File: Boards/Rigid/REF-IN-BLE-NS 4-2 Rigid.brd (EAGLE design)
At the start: 44 x 96.5 mm, 82 parts, among them U1 NRF52832_10QFN48, U2 AEM10941, X1 32 MHz, X2 32.768 kHz

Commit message: Removed internal pullups, changed xtal caps 12pf
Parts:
- C1, C17, C18, C2: value 9pF -> 12pF
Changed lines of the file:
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@@
 <elements>
 <element name="AE1" library="00_PF_Nordic" package="BLE_ANTENNA_NORDIC_FLIPPED" value="2.4GHZ_ANTENNAFLIPPED" x="37.375" y="13.3" smashed="yes" rot="R270"/>
-<element name="C1" library="resistor" package="C0603" value="9pF" x="35.2" y="19.81" smashed="yes" rot="R90">
+<element name="C1" library="resistor" package="C0603" value="12pF" x="35.2" y="19.81" smashed="yes" rot="R90">
 <attribute name="NAME" x="35.765" y="18.775" size="1" layer="25" font="vector" rot="R90"/>
 <attribute name="VALUE" value="12pF" x="37.105" y="19.175" size="1.27" layer="27" rot="R90"/>
@@
 <attribute name="MFG_PART#" value="CL10A105KP8NNNC " x="28.31" y="17.19" size="1.778" layer="27" rot="R90" display="off"/>
 </element>
-<element name="C2" library="resistor" package="C0603" value="9pF" x="32.9" y="19.8" smashed="yes">
+<element name="C2" library="resistor" package="C0603" value="12pF" x="32.9" y="19.8" smashed="yes">
 <attribute name="NAME" x="32.065" y="19.335" size="1" layer="25" font="vector"/>
 <attribute name="VALUE" value="12pF" x="32.265" y="17.895" size="1.27" layer="27"/>
@@
 <attribute name="MFG_PART#" value="" x="20.5" y="20.2" size="1.778" layer="28" rot="MR180" display="off"/>
 </element>
-<element name="C17" library="resistor" package="C0603" value="9pF" x="20.71" y="14.63" smashed="yes" rot="R90">
+<element name="C17" library="resistor" package="C0603" value="12pF" x="20.71" y="14.63" smashed="yes" rot="R90">
 <attribute name="PERCENTAGE" value="5%" x="20.71" y="14.63" size="1.778" layer="27" rot="R90" display="off"/>
 <attribute name="MFG_PART#" value="C0603C120J5GACTU" x="20.71" y="14.63" size="1.778" layer="27" rot="R90" display="off"/>
@@
 <attribute name="VALUE" x="20.865" y="13.745" size="0.7" layer="27" font="vector" rot="R90"/>
 </element>
-<element name="C18" library="resistor" package="C0603" value="9pF" x="20.69" y="11.42" smashed="yes" rot="R270">
+<element name="C18" library="resistor" package="C0603" value="12pF" x="20.69" y="11.42" smashed="yes" rot="R270">
 <attribute name="PERCENTAGE" value="5%" x="20.69" y="11.42" size="1.778" layer="27" rot="R270" display="off"/>
 <attribute name="MFG_PART#" value="C0603C120J5GACTU" x="20.69" y="11.42" size="1.778" layer="27" rot="R270" display="off"/>

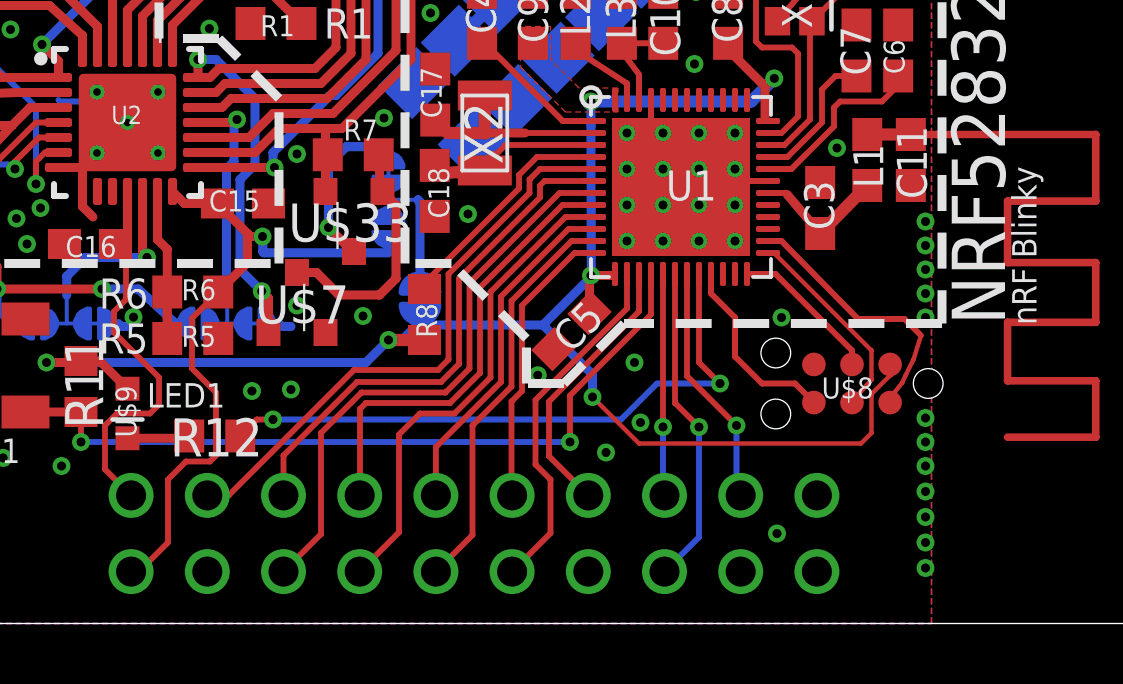
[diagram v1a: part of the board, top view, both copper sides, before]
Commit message: Finalized rigid & flex and code
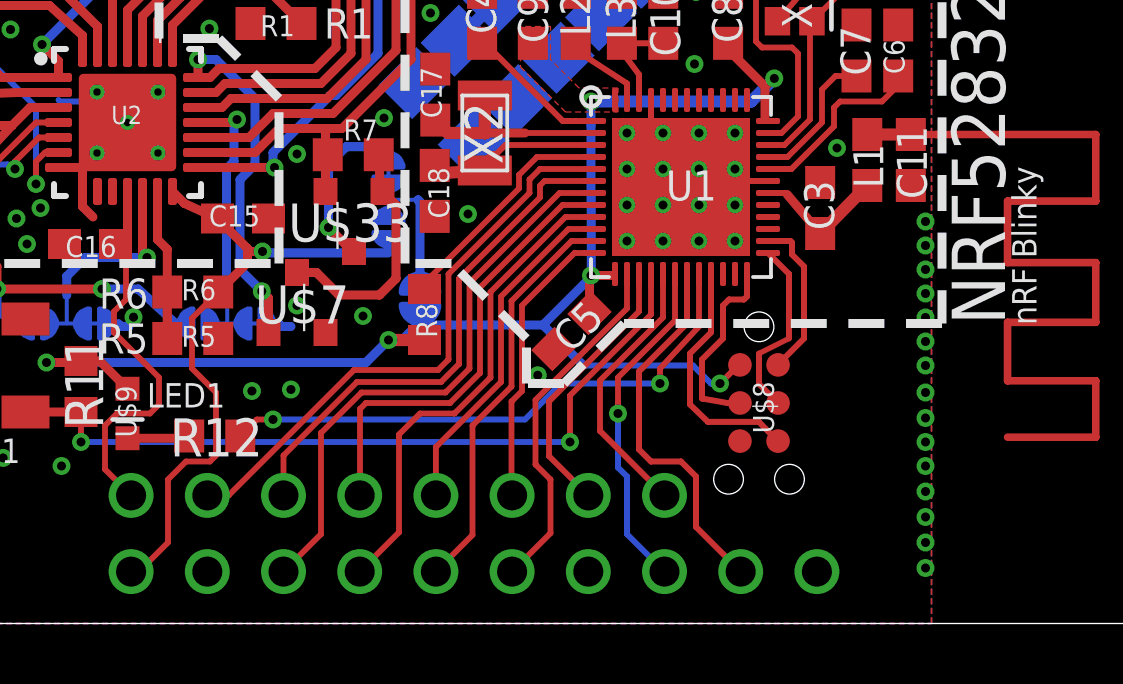
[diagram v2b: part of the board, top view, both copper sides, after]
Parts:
- C17, C18: value 12pF -> 12p
- U$20: value 20PIN_CONN -> 18PIN_CONN
- moved U$8 3.17 mm to (31.5, 4.35), turned to 270 degrees
- moved C15 0.50 mm to (14.3, 10.5)
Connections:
- net GND: no longer U$20.P$20, U$20.P$9
- net P16: now also U$20.P$9; no longer U$20.P$19
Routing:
- net HVOUT: track 59.4 -> 50.9 mm
- net P16: track 8.12 -> 12.6 mm, vias 1 -> 0
- net N$24: track 8.92 -> 5.42 mm
- net P14: track 7.40 -> 9.21 mm, vias 1 -> 0
- net N$31: track 20.7 -> 18.9 mm
- net N$25: track 6.35 -> 8.08 mm
- net N$22: track 5.02 -> 6.34 mm
- net PREHV: track 22.8 -> 21.6 mm
- net P15: track 10.7 -> 11.3 mm
- net N$21: track 6.78 -> 6.17 mm
- net GND: vias 76 -> 74
